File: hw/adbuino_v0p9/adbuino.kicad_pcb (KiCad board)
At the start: 2 copper layers, 30.7 x 50 mm, 22 parts, among them IC1 MAX3421EEHJ+, J1 U254-051N-4BH806, J2 USB_A, J3 Mini-DIN-4, J4 Mini-DIN-4, SW1 SW_Push, U1 ATmega328P-AU, U2 AMS1117-3.3

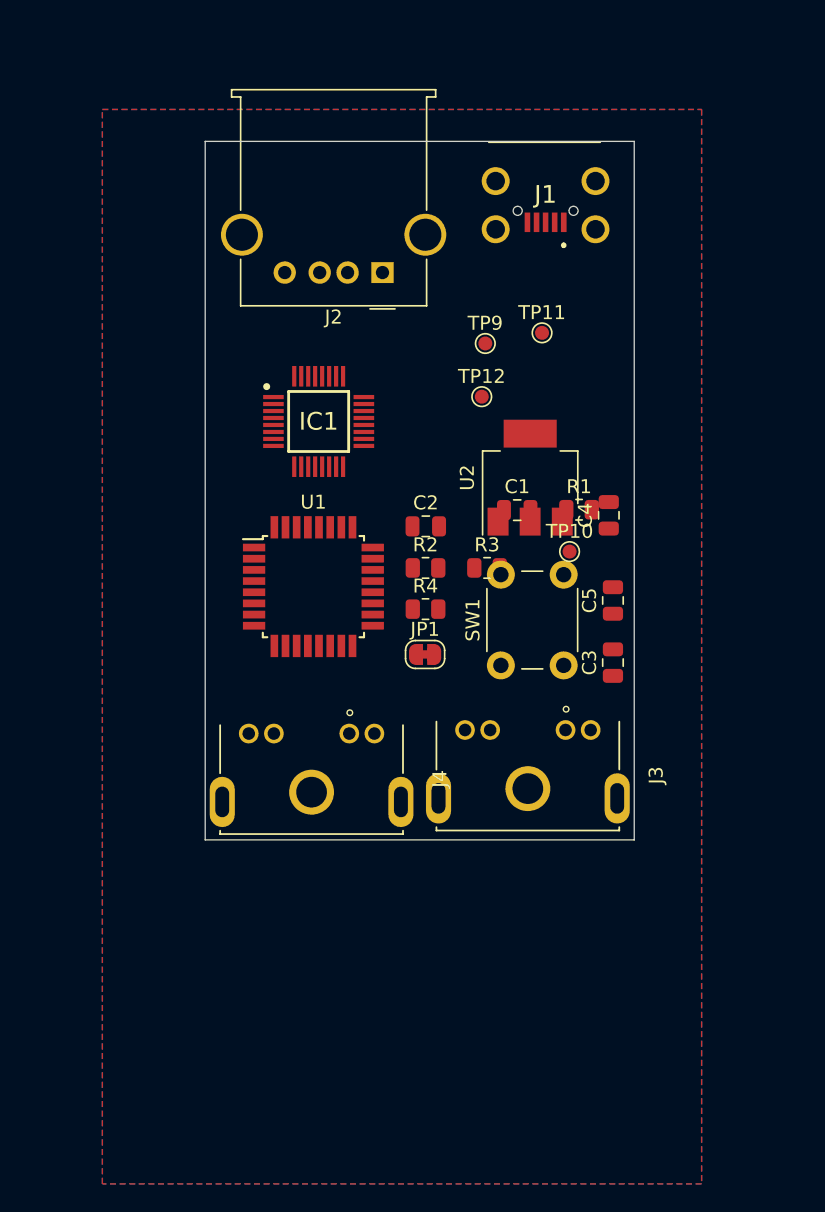
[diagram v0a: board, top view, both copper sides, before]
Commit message: Finished initial board layout
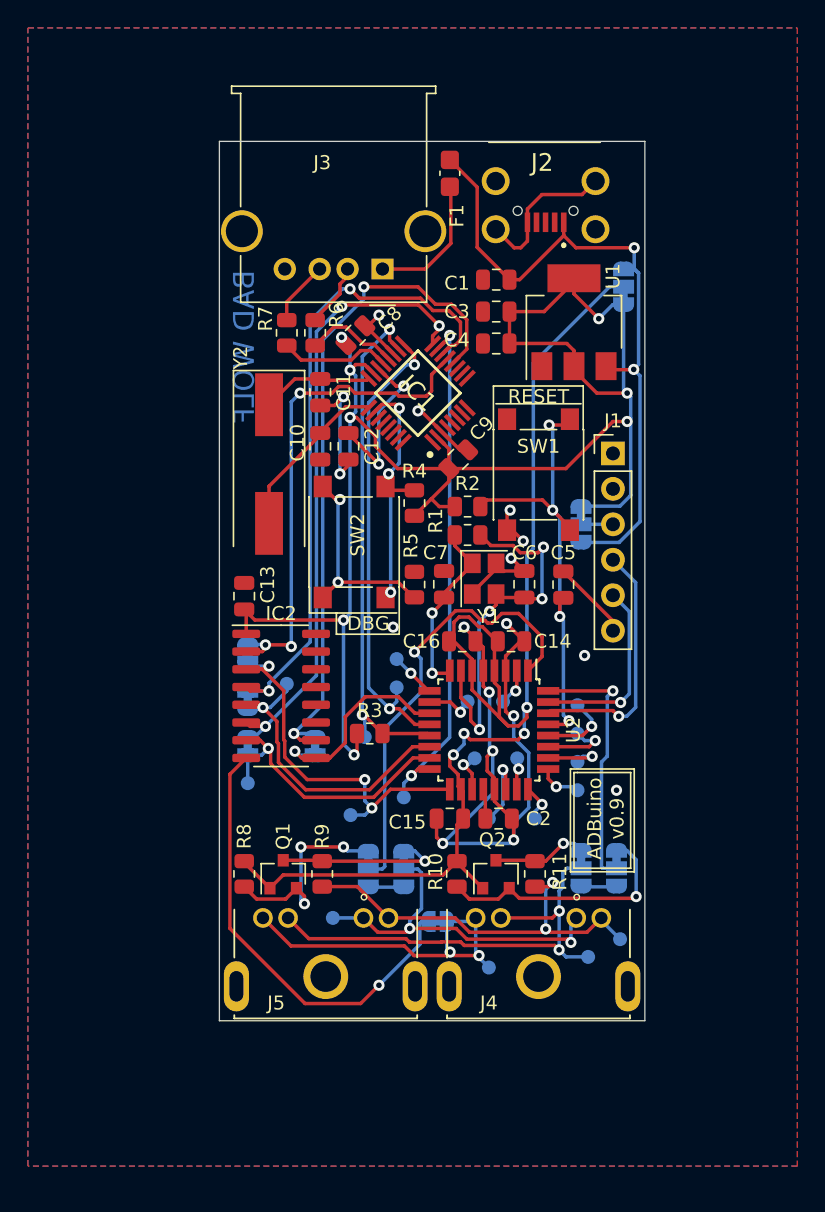
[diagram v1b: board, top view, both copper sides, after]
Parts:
- removed the C3 at (182.1, 73.9)
- removed the J3 at (176.0, 82.0)
- added C10: 30p, Capacitor_SMD:C_0805_2012Metric, F.Cu at (161.2, 58.4)
- added C11: 30p, Capacitor_SMD:C_0805_2012Metric, F.Cu at (161.2, 54.5)
- added C12: 100n, Capacitor_SMD:C_0805_2012Metric, F.Cu at (163.2, 58.4)
- added C13: 100n, Capacitor_SMD:C_0805_2012Metric, F.Cu at (155.7, 69.2)
- added C14: 100n, Capacitor_SMD:C_0805_2012Metric, F.Cu at (174.8, 72.4)
- added C15: 100n, Capacitor_SMD:C_0805_2012Metric, F.Cu at (170.4, 85.1)
- added C16: 100n, Capacitor_SMD:C_0805_2012Metric, F.Cu at (171.3, 72.4)
- added C2: 100n, Capacitor_SMD:C_0805_2012Metric, F.Cu at (173.9, 85.1)
- added C5: 100n, Capacitor_SMD:C_0805_2012Metric, F.Cu at (178.6, 68.3)
- added C6: 4p, Capacitor_SMD:C_0805_2012Metric, F.Cu at (175.8, 68.3)
- added C7: 4p, Capacitor_SMD:C_0805_2012Metric, F.Cu at (170.0, 68.3)
- added C8: 100n, Capacitor_SMD:C_0805_2012Metric, F.Cu at (163.7, 50.5)
- added F1: Polyfuse, Fuse:Fuse_0805_2012Metric_Castellated, F.Cu at (170.4, 38.9)
- added IC2: 74HC4050D,653, Package_SO:SOP-16_3.9x9.9mm_P1.27mm, F.Cu at (158.3, 76.3)
- added J1: Conn_01x06_Male, Connector_PinHeader_2.54mm:PinHeader_1x06_P2.54mm_Vertical, F.Cu at (182.1, 58.9)
- added J4: Mini-DIN-4, adbuino_v0p1:CUI_MD2-40ST, F.Cu at (176.8, 95.5)
- added JP1: SolderJumper_3_Bridged12, Jumper:SolderJumper-3_P1.3mm_Bridged12_RoundedPad1.0x1.5mm_NumberLabels, B.Cu at (179.8, 64.0)
- added JP10: SolderJumper_3_Bridged12, Jumper:SolderJumper-3_P1.3mm_Bridged12_RoundedPad1.0x1.5mm_NumberLabels, B.Cu at (182.4, 88.6)
- added JP11: SolderJumper_3_Bridged12, Jumper:SolderJumper-3_P1.3mm_Bridged12_RoundedPad1.0x1.5mm_NumberLabels, B.Cu at (179.8, 88.6)
- added JP2: SolderJumper_3_Bridged12, Jumper:SolderJumper-3_P1.3mm_Bridged12_RoundedPad1.0x1.5mm_NumberLabels, B.Cu at (182.9, 47.0)
- added JP3: SolderJumper_2_Bridged, Jumper:SolderJumper-2_P1.3mm_Bridged_RoundedPad1.0x1.5mm, B.Cu at (160.8, 79.9)
- added JP4: SolderJumper_2_Bridged, Jumper:SolderJumper-2_P1.3mm_Bridged_RoundedPad1.0x1.5mm, B.Cu at (156.0, 73.3)
- added JP5: SolderJumper_2_Bridged, Jumper:SolderJumper-2_P1.3mm_Bridged_RoundedPad1.0x1.5mm, B.Cu at (156.0, 76.6)
- added JP6: SolderJumper_2_Bridged, Jumper:SolderJumper-2_P1.3mm_Bridged_RoundedPad1.0x1.5mm, B.Cu at (156.0, 79.9)
- added JP8: SolderJumper_3_Bridged12, Jumper:SolderJumper-3_P1.3mm_Bridged12_RoundedPad1.0x1.5mm_NumberLabels, B.Cu at (164.6, 88.7)
- added JP9: SolderJumper_3_Bridged12, Jumper:SolderJumper-3_P1.3mm_Bridged12_RoundedPad1.0x1.5mm_NumberLabels, B.Cu at (167.1, 88.7)
- added Q1: BSS138, Package_TO_SOT_SMD:SOT-23, F.Cu at (158.5, 89.1)
- added Q2: BSS138, Package_TO_SOT_SMD:SOT-23, F.Cu at (173.7, 89.1)
- added R1: 1M, Resistor_SMD:R_0805_2012Metric, F.Cu at (171.7, 64.8)
- added R10: 10k, Resistor_SMD:R_0805_2012Metric, F.Cu at (170.9, 89.1)
- added R11: 10k, Resistor_SMD:R_0805_2012Metric, F.Cu at (176.5, 89.1)
- added R2: 10k, Resistor_SMD:R_0805_2012Metric, F.Cu at (171.7, 62.7)
- added R3: 2.2k, Resistor_SMD:R_0805_2012Metric, F.Cu at (164.7, 79.0)
- added R8: 10k, Resistor_SMD:R_0805_2012Metric, F.Cu at (155.7, 89.1)
- added R9: 10k, Resistor_SMD:R_0805_2012Metric, F.Cu at (161.3, 89.1)
- added SW1: SW_Push, Button_Switch_SMD:SW_Push_1P1T_NO_6x6mm_H9.5mm, F.Cu at (176.8, 60.5)
- added TP1: TestPoint_Small, TestPoint:TestPoint_Pad_D1.0mm, B.Cu at (172.2, 80.8)
- added TP10: TestPoint_Small, TestPoint:TestPoint_Pad_D1.0mm, B.Cu at (176.5, 85.1)
- added TP12: TestPoint_Small, TestPoint:TestPoint_Pad_D1.0mm, B.Cu at (179.6, 81.0)
- added TP13: TestPoint_Small, TestPoint:TestPoint_Pad_D1.0mm, B.Cu at (179.6, 79.0)
- added TP14: TestPoint_Small, TestPoint:TestPoint_Pad_D1.0mm, B.Cu at (179.6, 77.0)
- added TP15: TestPoint_Small, TestPoint:TestPoint_Pad_D1.0mm, B.Cu at (174.2, 76.7)
- added TP16: TestPoint_Small, TestPoint:TestPoint_Pad_D1.0mm, B.Cu at (166.6, 73.7)
- added TP17: TestPoint_Small, TestPoint:TestPoint_Pad_D1.0mm, B.Cu at (171.7, 76.7)
- added TP2: TestPoint_Small, TestPoint:TestPoint_Pad_D1.0mm, B.Cu at (173.2, 85.1)
- added TP20: TestPoint_Small, TestPoint:TestPoint_Pad_D1.0mm, B.Cu at (182.6, 93.7)
- added TP3: TestPoint_Small, TestPoint:TestPoint_Pad_D1.0mm, B.Cu at (166.6, 75.7)
- added TP4: TestPoint_Small, TestPoint:TestPoint_Pad_D1.0mm, B.Cu at (164.3, 79.2)
- added TP5: TestPoint_Small, TestPoint:TestPoint_Pad_D1.0mm, B.Cu at (158.8, 75.4)
- added TP6: TestPoint_Small, TestPoint:TestPoint_Pad_D1.0mm, B.Cu at (156.0, 82.5)
- added TP7: TestPoint_Small, TestPoint:TestPoint_Pad_D1.0mm, B.Cu at (167.1, 83.6)
- added TP8: TestPoint_Small, TestPoint:TestPoint_Pad_D1.0mm, B.Cu at (163.3, 84.8)
- added TP9: TestPoint_Small, TestPoint:TestPoint_Pad_D1.0mm, B.Cu at (175.3, 80.8)
- added Y1: 16MHz, Crystal:Crystal_SMD_3225-4Pin_3.2x2.5mm, F.Cu at (172.9, 67.9)
- added Y2: 12MHz, Crystal:Crystal_SMD_HC49-SD, F.Cu at (157.5, 59.7)
- C1: value 100n -> 10u
- JP7: renamed from JP1; moved to B.Cu
- SW2: renamed from SW1; footprint Button_Switch_THT:SW_PUSH_6mm -> Button_Switch_SMD:SW_Push_1P1T_NO_6x6mm_H9.5mm
- TP11: moved to B.Cu
- TP18: renamed from TP9; moved to B.Cu
- TP19: renamed from TP10; moved to B.Cu
- TP21: renamed from TP12; moved to B.Cu
- moved TP18 42.6 mm to (162.1, 92.2)
- moved TP21 40.9 mm to (173.2, 95.8)
- moved TP11 32.9 mm to (179.6, 83.1), turned to 270 degrees
- moved TP19 29.1 mm to (180.3, 95.0)
- moved R7 22.1 mm to (158.8, 50.3), turned to 90 degrees
- moved R6 20.9 mm to (160.8, 50.3), turned to 270 degrees
- moved C4 20.2 mm to (173.8, 51.1), turned to 180 degrees
- moved JP7 19.1 mm to (169.6, 92.5)
- moved C3 16.7 mm to (173.8, 48.8), turned to 180 degrees
- moved C1 16.6 mm to (173.8, 46.5), turned to 180 degrees
- moved U2 16.2 mm to (173.2, 78.7), turned to 270 degrees
- moved SW2 13.7 mm to (163.6, 65.3), turned to 270 degrees
- moved J5 13.2 mm to (161.5, 95.5)
- moved R4 11.8 mm to (167.9, 62.5), turned to 270 degrees
- moved U1 11.6 mm to (179.3, 49.5)
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- renumbered C4 to C3, C5 to C4, C2 to C9, J1 to J2, J2 to J3, J4 to J5, R1 to R4, R2 to R5, R3 to R6, R4 to R7, U2 to U1, U1 to U2
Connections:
- C1 pad 1: +3V3 -> VBUS
- IC1 pad 12: (no net) -> MAX3421_RESET
- IC1 pad 13: (no net) -> SPI_SCLK
- IC1 pad 14: (no net) -> MAX3421_SS
- IC1 pad 15: (no net) -> SPI_MISO
- IC1 pad 16: (no net) -> SPI_MOSI
- IC1 pad 17: (no net) -> MAX3421_GPX
- IC1 pad 18: (no net) -> MAX3421_INT
- IC1 pad 22: (no net) -> Net-(C12-Pad1)
- IC1 pad 24: (no net) -> Net-(C11-Pad1)
- IC1 pad 25: (no net) -> Net-(C10-Pad1)
- J3 pad 1: VBUS -> Net-(F1-Pad1)
- TP11 pad 1: ADB_1_5v -> Net-(TP11-Pad1)
- U2 pad 1: (no net) -> ADB_DATA_LV
- U2 pad 10: (no net) -> Net-(TP17-Pad1)
- U2 pad 11: (no net) -> TTL_MAX3421_RESET
- U2 pad 12: (no net) -> MAX3421_GPX
- U2 pad 13: (no net) -> MAX3421_INT
- U2 pad 14: (no net) -> TTL_SS
- U2 pad 15: (no net) -> TTL_SPI_MOSI
- U2 pad 16: (no net) -> SPI_MISO
- U2 pad 17: (no net) -> TTL_SPI_SCLK
- U2 pad 18: +3V3 -> VCC
- U2 pad 19: (no net) -> Net-(TP1-Pad1)
- U2 pad 2: (no net) -> Net-(TP15-Pad1)
- U2 pad 20: (no net) -> Net-(C2-Pad1)
- U2 pad 22: (no net) -> Net-(TP2-Pad1)
- U2 pad 23: (no net) -> Net-(TP9-Pad1)
- U2 pad 24: (no net) -> Net-(TP10-Pad1)
- U2 pad 25: (no net) -> Net-(TP11-Pad1)
- U2 pad 26: (no net) -> Net-(TP12-Pad1)
- U2 pad 27: (no net) -> Net-(TP13-Pad1)
- U2 pad 28: (no net) -> Net-(TP14-Pad1)
- U2 pad 29: (no net) -> Net-(C5-Pad1)
- U2 pad 30: (no net) -> FTDI_RXI
- U2 pad 31: (no net) -> FTDI_TXO
- U2 pad 32: (no net) -> ADB_PWR_ON_LV
- U2 pad 4: +3V3 -> VCC
- U2 pad 6: +3V3 -> VCC
- U2 pad 7: (no net) -> Net-(C6-Pad1)
- U2 pad 8: (no net) -> Net-(C7-Pad1)
- U2 pad 9: (no net) -> Net-(TP16-Pad1)
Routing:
- net GND: track 0.00 -> 121.7 mm, vias 0 -> 18
- net +3V3: track 0.00 -> 118.7 mm, vias 0 -> 8
- net VCC: track 0.00 -> 92.1 mm, vias 0 -> 4
- net VBUS: track 0.00 -> 50.0 mm, vias 0 -> 2
- net MAX3421_RESET: track 0.00 -> 49.4 mm, vias 0 -> 2
- net MAX3421_SS: track 0.00 -> 46.7 mm, vias 0 -> 2
- net SPI_MOSI: track 0.00 -> 44.6 mm, vias 0 -> 3
- net SPI_MISO: track 0.00 -> 37.3 mm, vias 0 -> 2
- net MAX3421_INT: track 0.00 -> 37.2 mm, vias 0 -> 2
- net SPI_SCLK: track 0.00 -> 36.4 mm, vias 0 -> 3
- net Net-(C5-Pad1): track 0.00 -> 34.3 mm, vias 0 -> 4
- net ADB_1_PWR_ON: track 0.00 -> 34.2 mm, vias 0 -> 2
- net MAX3421_GPX: track 0.00 -> 33.8 mm, vias 0 -> 2
- net ADB_DATA_LV: track 0.00 -> 32.4 mm, vias 0 -> 1
- net ADB_1_5v: track 0.00 -> 29.0 mm, vias 0 -> 2
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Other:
- board size 30.7 x 50 mm -> 30.5 x 63 mm
- board text added: "ADB Port 1"
- board text added: "ADB Port 2"
- board text added: "ADBuino v0.9"
- board text added: "BAD WOLF"
- board text added: "DBG"
- board text added: "DTR"
- board text added: "GND"
- board text added: "PWR"
- board text added: "Power"
- board text added: "RESET"
- board text added: "RXI"
- board text added: "TXO"
- board text added: "USB Keyboard / Mouse"
- board text added: "https://github.com/akuker/adbuino"
